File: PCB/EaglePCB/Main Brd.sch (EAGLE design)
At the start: 70 parts, among them J2 702461401, U1 ATWINC1500-MR210PB1952-T, U3 MSP430FR2355TDBTRDBT0038A_M, U6 ARJM11C7-114-BA-EW2

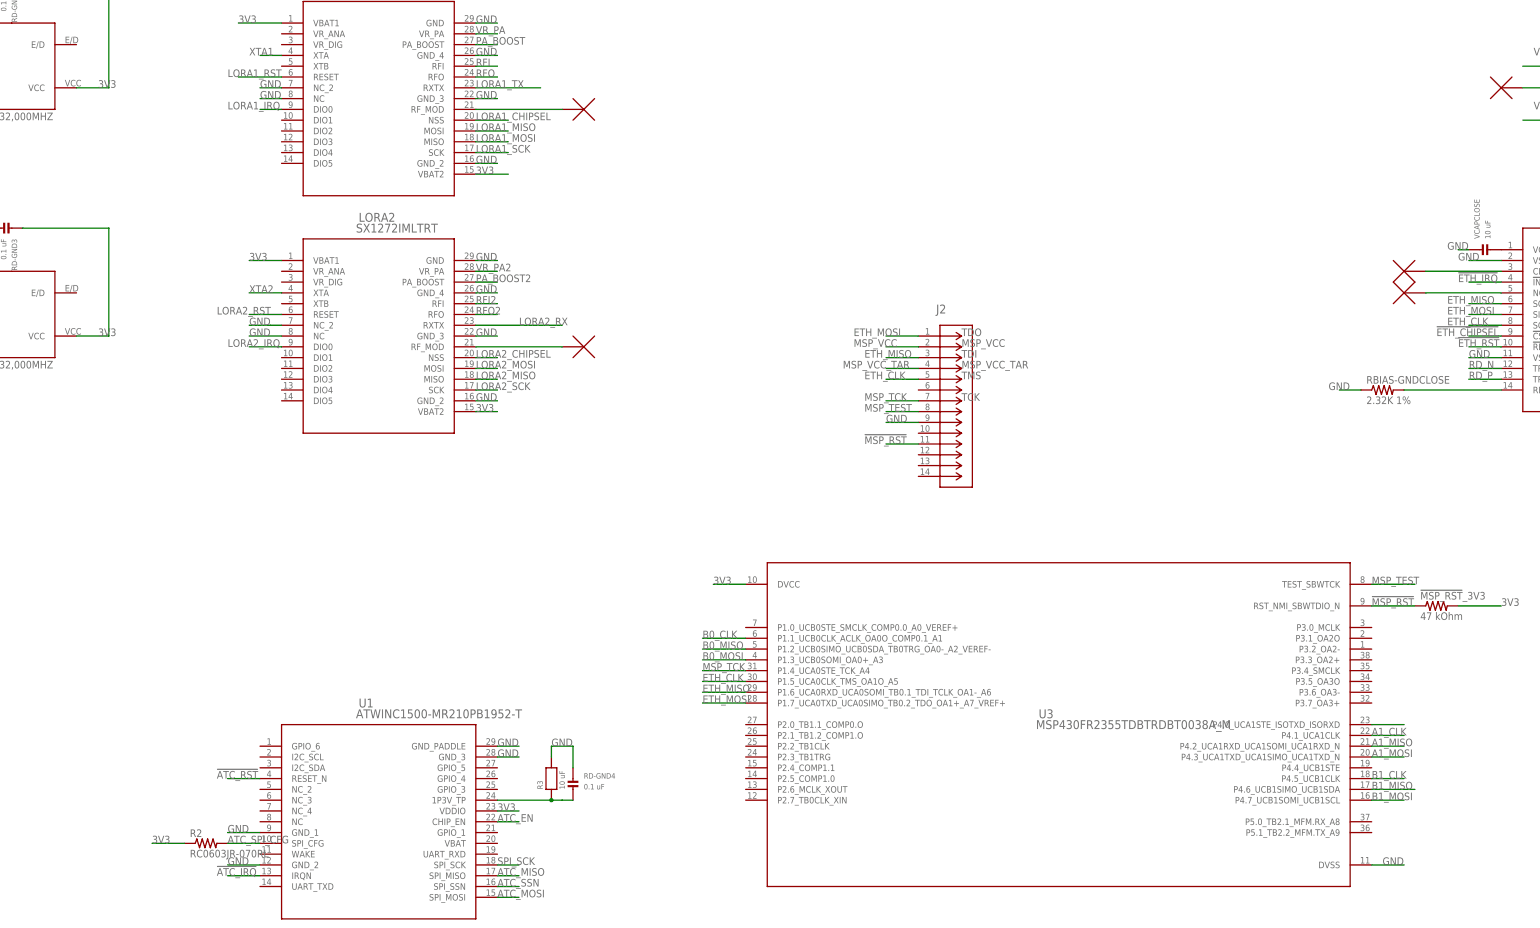
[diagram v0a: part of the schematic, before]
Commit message: pcb moving forward
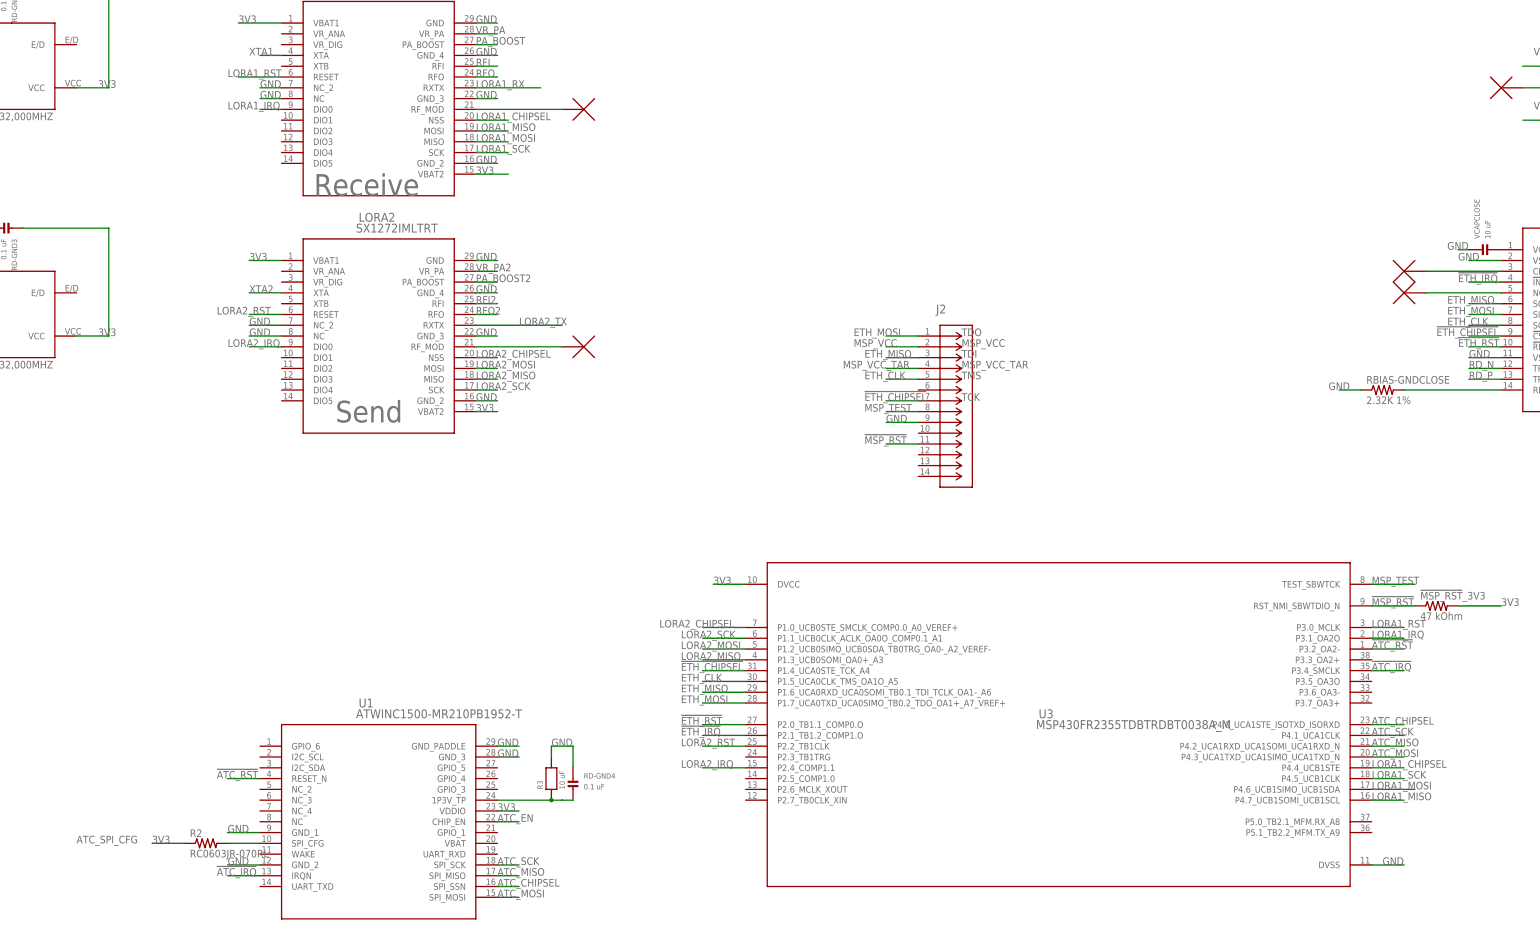
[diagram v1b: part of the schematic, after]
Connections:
- net LORA1_TX renamed LORA1_RX
- net LORA2_RX renamed LORA2_TX
- removed net A1_CLK: U3.P4.1_UCA1CLK
- removed net A1_MISO: U3.P4.2_UCA1RXD_UCA1SOMI_UCA1RXD_N
- removed net A1_MOSI: U3.P4.3_UCA1TXD_UCA1SIMO_UCA1TXD_N
- removed net ATC_SSN: U1.SPI_SSN
- removed net B0_CLK: U3.P1.1_UCB0CLK_ACLK_OA0O_COMP0.1_A1
- removed net B0_MISO: U3.P1.2_UCB0SIMO_UCB0SDA_TB0TRG_OA0-_A2_VEREF-
- removed net B0_MOSI: U3.P1.3_UCB0SOMI_OA0+_A3
- removed net B1_CLK: U3.P4.5_UCB1CLK
- removed net B1_MISO: U3.P4.6_UCB1SIMO_UCB1SDA
- removed net B1_MOSI: U3.P4.7_UCB1SOMI_UCB1SCL
- removed net MSP_TCK: J2.7, U3.P1.4_UCA0STE_TCK_A4
- removed net N$21: U3.P4.0_UCA1STE_ISOTXD_ISORXD
- removed net SPI_SCK: U1.SPI_SCK
- new net ATC_CHIPSEL: U1.SPI_SSN, U3.P4.0_UCA1STE_ISOTXD_ISORXD
- new net ATC_SCK: U1.SPI_SCK, U3.P4.1_UCA1CLK
- net !ATC_IRQ: now also U3.P3.4_SMCLK
- net !ATC_RST: now also U3.P3.2_OA2-
- net !ETH_CHIPSEL: now also J2.7, U3.P1.4_UCA0STE_TCK_A4
- net !ETH_IRQ: now also U3.P2.1_TB1.2_COMP1.O
- net !ETH_RST: now also U3.P2.0_TB1.1_COMP0.O
- net ATC_MISO: now also U3.P4.2_UCA1RXD_UCA1SOMI_UCA1RXD_N
- net ATC_MOSI: now also U3.P4.3_UCA1TXD_UCA1SIMO_UCA1TXD_N
- net LORA1_CHIPSEL: now also U3.P4.4_UCB1STE
- net LORA1_IRQ: now also U3.P3.1_OA2O
- net LORA1_MISO: now also U3.P4.7_UCB1SOMI_UCB1SCL
- net LORA1_MOSI: now also U3.P4.6_UCB1SIMO_UCB1SDA
- net LORA1_RST: now also U3.P3.0_MCLK
- net LORA1_SCK: now also U3.P4.5_UCB1CLK
- net LORA2_CHIPSEL: now also U3.P1.0_UCB0STE_SMCLK_COMP0.0_A0_VEREF+
- net LORA2_IRQ: now also U3.P2.4_COMP1.1
- net LORA2_MISO: now also U3.P1.3_UCB0SOMI_OA0+_A3
- net LORA2_MOSI: now also U3.P1.2_UCB0SIMO_UCB0SDA_TB0TRG_OA0-_A2_VEREF-
- net LORA2_RST: now also U3.P2.2_TB1CLK
- net LORA2_SCK: now also U3.P1.1_UCB0CLK_ACLK_OA0O_COMP0.1_A1
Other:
- note added: "Receive"
- note added: "Send"
